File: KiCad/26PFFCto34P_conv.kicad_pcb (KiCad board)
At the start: 2 copper layers, 50 x 18 mm, 7 parts, among them J1 FDD, J2 FDC, J3 -+, J4 Conn_01x03, J5 Conn_01x03

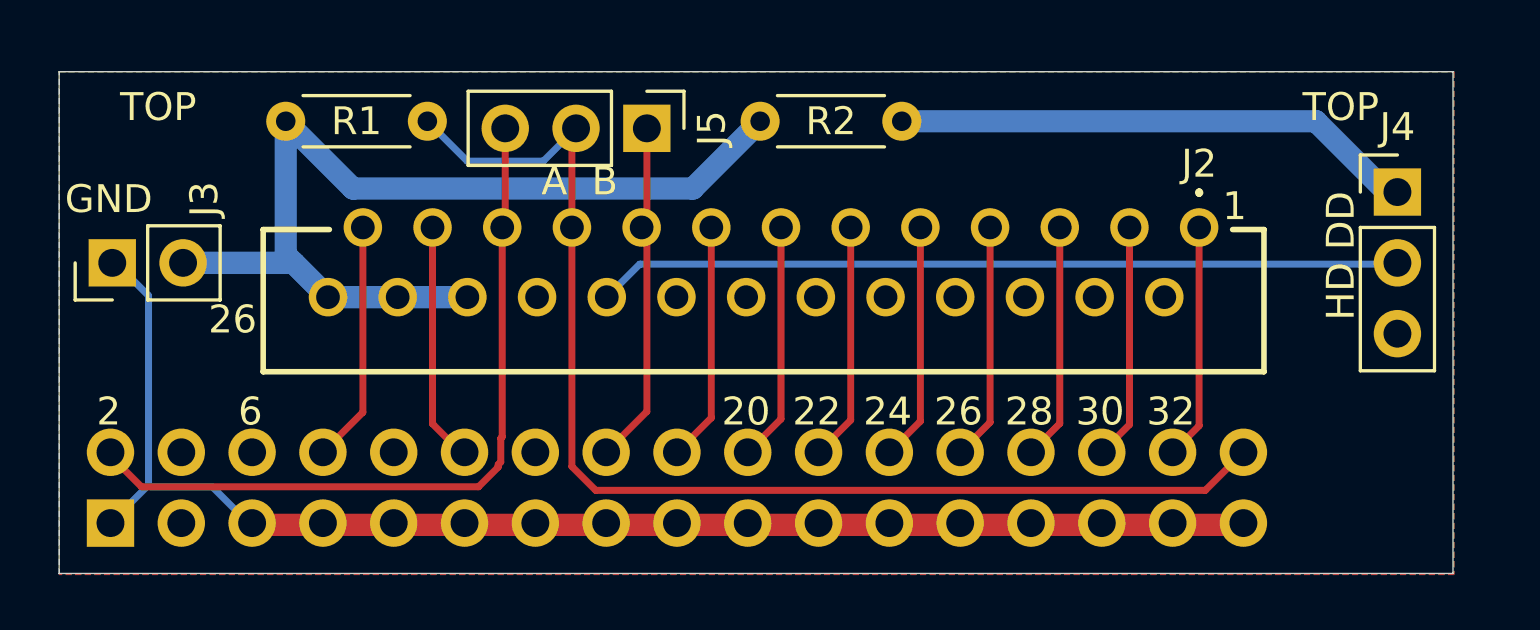
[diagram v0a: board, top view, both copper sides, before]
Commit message: Further miniaturization
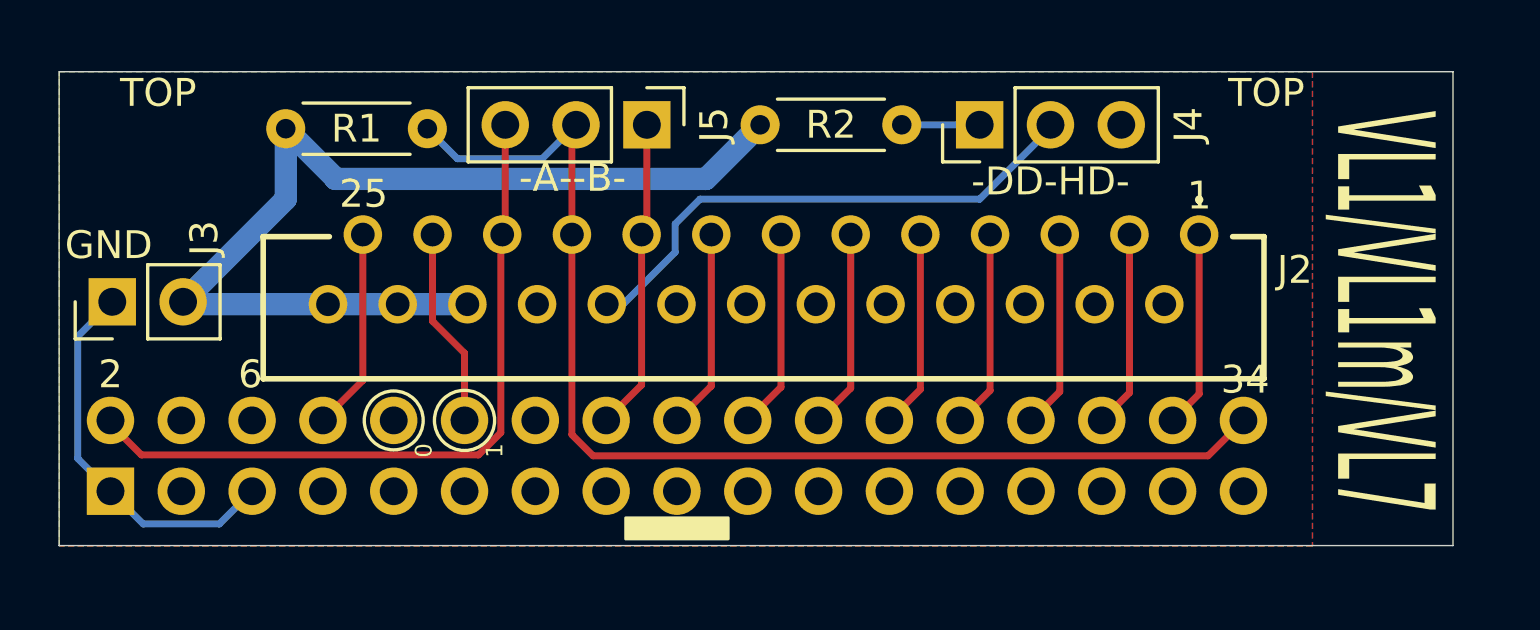
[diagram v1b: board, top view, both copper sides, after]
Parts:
- J2: footprint kicad_by_BakudaLab:morex520452645 -> 26PFFCto34P_conv:morex520452645
- moved J4 15.2 mm to (83.8, 52.7), turned to 90 degrees
- moved J3 1.40 mm to (52.7, 59.1)
- moved J1 1.14 mm to (52.6, 65.8)
- moved R1 0.27 mm to (58.9, 52.8)
- moved J2 0.25 mm to (91.7, 56.6)
- moved J5 0.13 mm to (71.9, 52.7)
- moved R2 0.13 mm to (75.9, 52.7)
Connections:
- net /DIR# renamed /DIR
- net /DISKCHANGE# renamed /DISKCHANGE
- net /DS1# renamed /DRIVESELECT
- net /INDEX# renamed /INDEX
- net /READDATA# renamed /READDATA
- net /READY# renamed /READY
- net /STEP# renamed /STEP
- net /TRACK00# renamed /TRACK00
- net /WRITEDATA# renamed /WRITEDATA
- net /WRITEGATE# renamed /WRITEGATE
- net /WRITEPROTECT# renamed /WRITEPROTECT
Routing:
- net GND: track 50.9 -> 13.8 mm
- net Net-(J4-Pad1): track 18.8 -> 2.79 mm
- net /HDOUT#: track 28.9 -> 19.1 mm
- net /DRIVESELECT: track 8.58 -> 7.14 mm
- net /READY: track 43.6 -> 42.2 mm
- net /WRITEPROTECT: track 8.58 -> 7.18 mm
- net /WRITEGATE: track 8.62 -> 7.22 mm
- net /WRITEDATA: track 8.63 -> 7.23 mm
- net /READDATA: track 8.57 -> 7.17 mm
- net /INDEX: track 8.75 -> 7.35 mm
- net /TRACK00: track 8.60 -> 7.20 mm
- net /STEP: track 8.65 -> 7.25 mm
- net /SIDE1: track 8.55 -> 7.15 mm
- net /DIR: track 8.66 -> 7.27 mm
- net /MOTORON#: track 12.6 -> 11.3 mm
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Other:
- board size 50 x 18 mm -> 50 x 17 mm
- board text added: "-A--B-"
- board text added: "-DD-HD-"
- board text added: "0"
- board text added: "25"
- board text added: "26P FFC to 34P Shugart Version 0.1 by Bakuda Lab 2021"
- board text added: "34"
- board text added: "VL1/VL1m/VL7"
- board text removed: "20"
- board text removed: "22"
- board text removed: "24"
- board text removed: "26"
- board text removed: "28"
- board text removed: "30"
- board text removed: "32"
- board text removed: "A B"
- board text removed: "FFC 26P to 34P Version 0.1 by Bakuda Lab 2021"
- board text removed: "HD DD"
